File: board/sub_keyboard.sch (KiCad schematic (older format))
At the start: 30 parts, among them SW1001 SW_SPST, SW1002 SW_SPST, SW1003 SW_SPST, SW1004 SW_SPST, SW1005 SW_SPST, SW1006 SW_SPST, SW1007 SW_SPST, SW1008 SW_SPST, SW1009 SW_SPST, SW1010 SW_SPST, SW1011 SW_SPST, SW1012 SW_SPST, SW1013 SW_SPST, SW1014 SW_SPST, SW1015 SW_SPST, SW1016 SW_SPST, SW1017 SW_SPST, SW1018 SW_SPST, SW1019 SW_SPST, SW1020 SW_SPST, SW1021 SW_SPST, SW1022 SW_SPST, SW1023 SW_SPST, SW1024 SW_SPST, SW1025 SW_SPST, SW1026 SW_SPST, SW1027 SW_SPST, SW1028 SW_SPST, SW1029 SW_SPST, SW1030 SW_SPST

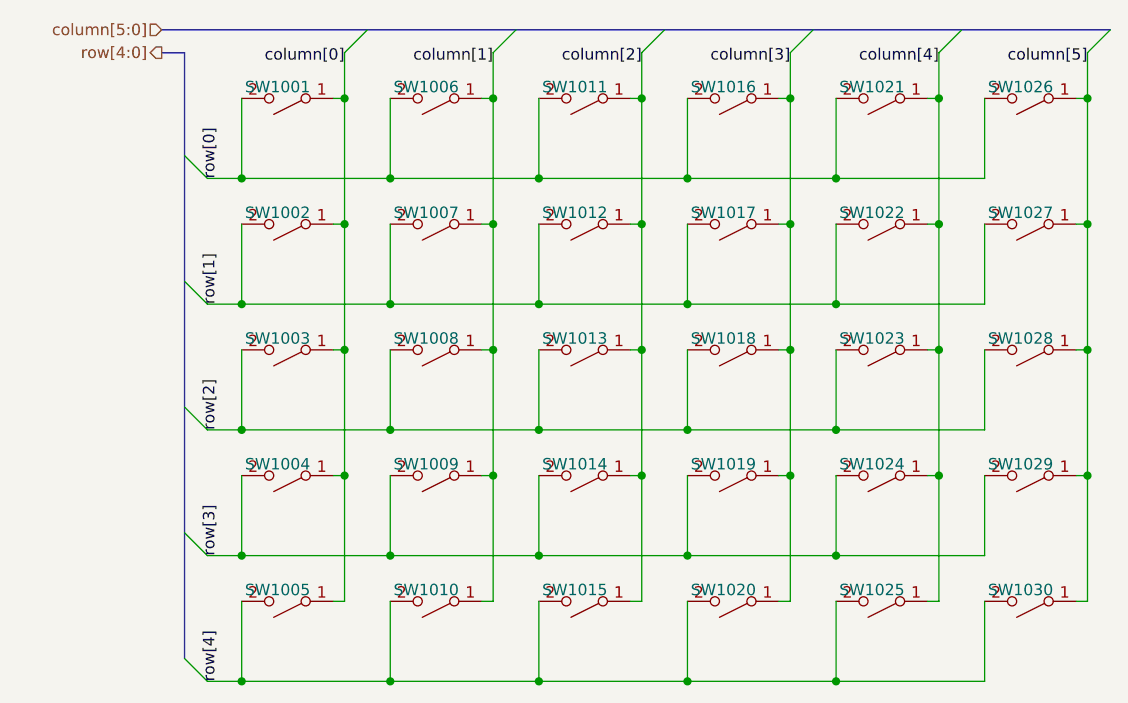
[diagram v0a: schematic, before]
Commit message: More Schematic progress
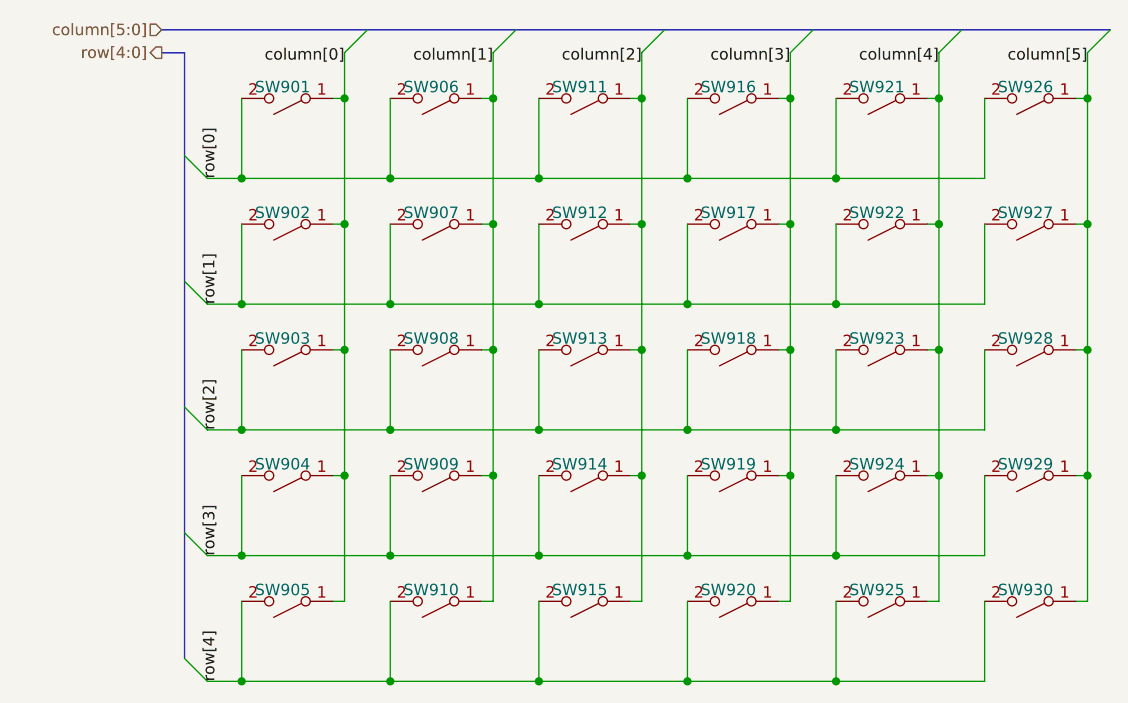
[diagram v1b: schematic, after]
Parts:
- renumbered SW1001 to SW901, SW1002 to SW902, SW1003 to SW903, SW1004 to SW904, SW1005 to SW905, SW1006 to SW906, SW1007 to SW907, SW1008 to SW908, SW1009 to SW909, SW1010 to SW910, SW1011 to SW911, SW1012 to SW912, SW1013 to SW913, SW1014 to SW914, SW1015 to SW915, SW1016 to SW916, SW1017 to SW917, SW1018 to SW918, SW1019 to SW919, SW1020 to SW920, SW1021 to SW921, SW1022 to SW922, SW1023 to SW923, SW1024 to SW924, SW1025 to SW925, SW1026 to SW926, SW1027 to SW927, SW1028 to SW928, SW1029 to SW929, SW1030 to SW930
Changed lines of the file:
@@
 $Descr A4 11693 8268
 encoding utf-8
-Sheet 10 15
+Sheet 9 14
 Title ""
 Date ""
@@
 row[4:0]
 $Comp
-L Switch:SW_SPST SW1001
+L Switch:SW_SPST SW901
 U 1 1 5A9DE7BF
 P 4600 2500
-F 0 "SW1001" H 4500 2450 50  0000 L CNN
+F 0 "SW901" H 4500 2450 50  0000 L CNN
 F 1 "SW_SPST" H 4450 2350 50  0001 L CNN
 F 2 "" H 4600 2500 50  0001 C CNN
@@
 $EndComp
 $Comp
-L Switch:SW_SPST SW1006
+L Switch:SW_SPST SW906
 U 1 1 5A9F6D51
 P 5250 2500
-F 0 "SW1006" H 5150 2450 50  0000 L CNN
+F 0 "SW906" H 5150 2450 50  0000 L CNN
 F 1 "SW_SPST" H 5100 2350 50  0001 L CNN
 F 2 "" H 5250 2500 50  0001 C CNN
@@
 $EndComp
 $Comp
-L Switch:SW_SPST SW1011
+L Switch:SW_SPST SW911
 U 1 1 5A9F724F
 P 5900 2500
-F 0 "SW1011" H 5800 2450 50  0000 L CNN
+F 0 "SW911" H 5800 2450 50  0000 L CNN
 F 1 "SW_SPST" H 5750 2350 50  0001 L CNN
 F 2 "" H 5900 2500 50  0001 C CNN
@@
 $EndComp
 $Comp
-L Switch:SW_SPST SW1016
+L Switch:SW_SPST SW916
 U 1 1 5A9F725B
 P 6550 2500
-F 0 "SW1016" H 6450 2450 50  0000 L CNN
+F 0 "SW916" H 6450 2450 50  0000 L CNN
 F 1 "SW_SPST" H 6400 2350 50  0001 L CNN
 F 2 "" H 6550 2500 50  0001 C CNN
@@
 $EndComp
 $Comp
-L Switch:SW_SPST SW1021
+L Switch:SW_SPST SW921
 U 1 1 5A9F738F
 P 7200 2500
-F 0 "SW1021" H 7100 2450 50  0000 L CNN
+F 0 "SW921" H 7100 2450 50  0000 L CNN
 F 1 "SW_SPST" H 7050 2350 50  0001 L CNN
 F 2 "" H 7200 2500 50  0001 C CNN
@@
 $EndComp
 $Comp
-L Switch:SW_SPST SW1026
+L Switch:SW_SPST SW926
 U 1 1 5A9F739B
 P 7850 2500
-F 0 "SW1026" H 7750 2450 50  0000 L CNN
+F 0 "SW926" H 7750 2450 50  0000 L CNN
 F 1 "SW_SPST" H 7700 2350 50  0001 L CNN
 F 2 "" H 7850 2500 50  0001 C CNN
@@
 $EndComp
 $Comp
-L Switch:SW_SPST SW1002
+L Switch:SW_SPST SW902
 U 1 1 5A9F7527
 P 4600 3050
-F 0 "SW1002" H 4500 3000 50  0000 L CNN
+F 0 "SW902" H 4500 3000 50  0000 L CNN
 F 1 "SW_SPST" H 4450 2900 50  0001 L CNN
 F 2 "" H 4600 3050 50  0001 C CNN
@@
 $EndComp
 $Comp
-L Switch:SW_SPST SW1007
+L Switch:SW_SPST SW907
 U 1 1 5A9F7533
 P 5250 3050
-F 0 "SW1007" H 5150 3000 50  0000 L CNN
+F 0 "SW907" H 5150 3000 50  0000 L CNN
 F 1 "SW_SPST" H 5100 2900 50  0001 L CNN
 F 2 "" H 5250 3050 50  0001 C CNN
@@
 $EndComp
 $Comp
-L Switch:SW_SPST SW1012
+L Switch:SW_SPST SW912
 U 1 1 5A9F753F
 P 5900 3050
-F 0 "SW1012" H 5800 3000 50  0000 L CNN
+F 0 "SW912" H 5800 3000 50  0000 L CNN
 F 1 "SW_SPST" H 5750 2900 50  0001 L CNN
 F 2 "" H 5900 3050 50  0001 C CNN
@@
 $EndComp
 $Comp
-L Switch:SW_SPST SW1017
+L Switch:SW_SPST SW917
 U 1 1 5A9F754B
 P 6550 3050
-F 0 "SW1017" H 6450 3000 50  0000 L CNN
+F 0 "SW917" H 6450 3000 50  0000 L CNN
 F 1 "SW_SPST" H 6400 2900 50  0001 L CNN
 F 2 "" H 6550 3050 50  0001 C CNN
@@
 $EndComp
 $Comp
-L Switch:SW_SPST SW1022
+L Switch:SW_SPST SW922
 U 1 1 5A9F7557
 P 7200 3050
-F 0 "SW1022" H 7100 3000 50  0000 L CNN
+F 0 "SW922" H 7100 3000 50  0000 L CNN
 F 1 "SW_SPST" H 7050 2900 50  0001 L CNN
 F 2 "" H 7200 3050 50  0001 C CNN
@@
 $EndComp
 $Comp
-L Switch:SW_SPST SW1027
+L Switch:SW_SPST SW927
 U 1 1 5A9F7563
 P 7850 3050
-F 0 "SW1027" H 7750 3000 50  0000 L CNN
+F 0 "SW927" H 7750 3000 50  0000 L CNN
 F 1 "SW_SPST" H 7700 2900 50  0001 L CNN
 F 2 "" H 7850 3050 50  0001 C CNN
@@
 $EndComp
 $Comp
-L Switch:SW_SPST SW1003
+L Switch:SW_SPST SW903
 U 1 1 5A9F8C97
 P 4600 3600
-F 0 "SW1003" H 4500 3550 50  0000 L CNN
+F 0 "SW903" H 4500 3550 50  0000 L CNN
 F 1 "SW_SPST" H 4450 3450 50  0001 L CNN
 F 2 "" H 4600 3600 50  0001 C CNN
@@
 $EndComp
 $Comp
-L Switch:SW_SPST SW1008
+L Switch:SW_SPST SW908
 U 1 1 5A9F8CA3
 P 5250 3600
-F 0 "SW1008" H 5150 3550 50  0000 L CNN
+F 0 "SW908" H 5150 3550 50  0000 L CNN
 F 1 "SW_SPST" H 5100 3450 50  0001 L CNN
 F 2 "" H 5250 3600 50  0001 C CNN
@@
 $EndComp
 $Comp
-L Switch:SW_SPST SW1013
+L Switch:SW_SPST SW913
 U 1 1 5A9F8CAF
 P 5900 3600
-F 0 "SW1013" H 5800 3550 50  0000 L CNN
+F 0 "SW913" H 5800 3550 50  0000 L CNN
 F 1 "SW_SPST" H 5750 3450 50  0001 L CNN
 F 2 "" H 5900 3600 50  0001 C CNN
@@
 $EndComp
 $Comp
-L Switch:SW_SPST SW1018
+L Switch:SW_SPST SW918
 U 1 1 5A9F8CBB
 P 6550 3600
-F 0 "SW1018" H 6450 3550 50  0000 L CNN
+F 0 "SW918" H 6450 3550 50  0000 L CNN
 F 1 "SW_SPST" H 6400 3450 50  0001 L CNN
 F 2 "" H 6550 3600 50  0001 C CNN
@@
 $EndComp
 $Comp
-L Switch:SW_SPST SW1023
+L Switch:SW_SPST SW923
 U 1 1 5A9F8CC7
 P 7200 3600
-F 0 "SW1023" H 7100 3550 50  0000 L CNN
+F 0 "SW923" H 7100 3550 50  0000 L CNN
 F 1 "SW_SPST" H 7050 3450 50  0001 L CNN
 F 2 "" H 7200 3600 50  0001 C CNN
@@
 $EndComp
 $Comp
-L Switch:SW_SPST SW1028
+L Switch:SW_SPST SW928
 U 1 1 5A9F8CD3
 P 7850 3600
-F 0 "SW1028" H 7750 3550 50  0000 L CNN
+F 0 "SW928" H 7750 3550 50  0000 L CNN
 F 1 "SW_SPST" H 7700 3450 50  0001 L CNN
 F 2 "" H 7850 3600 50  0001 C CNN
@@
 $EndComp
 $Comp
-L Switch:SW_SPST SW1004
+L Switch:SW_SPST SW904
 U 1 1 5A9F94D7
 P 4600 4150
-F 0 "SW1004" H 4500 4100 50  0000 L CNN
+F 0 "SW904" H 4500 4100 50  0000 L CNN
 F 1 "SW_SPST" H 4450 4000 50  0001 L CNN
 F 2 "" H 4600 4150 50  0001 C CNN
@@
 $EndComp
 $Comp
-L Switch:SW_SPST SW1009
+L Switch:SW_SPST SW909
 U 1 1 5A9F94E3
 P 5250 4150
-F 0 "SW1009" H 5150 4100 50  0000 L CNN
+F 0 "SW909" H 5150 4100 50  0000 L CNN
 F 1 "SW_SPST" H 5100 4000 50  0001 L CNN
 F 2 "" H 5250 4150 50  0001 C CNN
@@
 $EndComp
 $Comp
-L Switch:SW_SPST SW1014
+L Switch:SW_SPST SW914
 U 1 1 5A9F94EF
 P 5900 4150
-F 0 "SW1014" H 5800 4100 50  0000 L CNN
+F 0 "SW914" H 5800 4100 50  0000 L CNN
 F 1 "SW_SPST" H 5750 4000 50  0001 L CNN
 F 2 "" H 5900 4150 50  0001 C CNN
@@
 $EndComp
 $Comp
-L Switch:SW_SPST SW1019
+L Switch:SW_SPST SW919
 U 1 1 5A9F94FB
 P 6550 4150
-F 0 "SW1019" H 6450 4100 50  0000 L CNN
+F 0 "SW919" H 6450 4100 50  0000 L CNN
 F 1 "SW_SPST" H 6400 4000 50  0001 L CNN
 F 2 "" H 6550 4150 50  0001 C CNN
@@
 $EndComp
 $Comp
-L Switch:SW_SPST SW1024
+L Switch:SW_SPST SW924
 U 1 1 5A9F9507
 P 7200 4150
-F 0 "SW1024" H 7100 4100 50  0000 L CNN
+F 0 "SW924" H 7100 4100 50  0000 L CNN
 F 1 "SW_SPST" H 7050 4000 50  0001 L CNN
 F 2 "" H 7200 4150 50  0001 C CNN
@@
 $EndComp
 $Comp
-L Switch:SW_SPST SW1029
+L Switch:SW_SPST SW929
 U 1 1 5A9F9513
 P 7850 4150
-F 0 "SW1029" H 7750 4100 50  0000 L CNN
+F 0 "SW929" H 7750 4100 50  0000 L CNN
 F 1 "SW_SPST" H 7700 4000 50  0001 L CNN
 F 2 "" H 7850 4150 50  0001 C CNN
@@
 $EndComp
 $Comp
-L Switch:SW_SPST SW1005
+L Switch:SW_SPST SW905
 U 1 1 5A9F951F
 P 4600 4700
-F 0 "SW1005" H 4500 4650 50  0000 L CNN
+F 0 "SW905" H 4500 4650 50  0000 L CNN
 F 1 "SW_SPST" H 4450 4550 50  0001 L CNN
 F 2 "" H 4600 4700 50  0001 C CNN
@@
 $EndComp
 $Comp
-L Switch:SW_SPST SW1010
+L Switch:SW_SPST SW910
 U 1 1 5A9F952B
 P 5250 4700
-F 0 "SW1010" H 5150 4650 50  0000 L CNN
+F 0 "SW910" H 5150 4650 50  0000 L CNN
 F 1 "SW_SPST" H 5100 4550 50  0001 L CNN
 F 2 "" H 5250 4700 50  0001 C CNN
@@
 $EndComp
 $Comp
-L Switch:SW_SPST SW1015
+L Switch:SW_SPST SW915
 U 1 1 5A9F9537
 P 5900 4700
-F 0 "SW1015" H 5800 4650 50  0000 L CNN
+F 0 "SW915" H 5800 4650 50  0000 L CNN
 F 1 "SW_SPST" H 5750 4550 50  0001 L CNN
 F 2 "" H 5900 4700 50  0001 C CNN
@@
 $EndComp
 $Comp
-L Switch:SW_SPST SW1020
+L Switch:SW_SPST SW920
 U 1 1 5A9F9543
 P 6550 4700
-F 0 "SW1020" H 6450 4650 50  0000 L CNN
+F 0 "SW920" H 6450 4650 50  0000 L CNN
 F 1 "SW_SPST" H 6400 4550 50  0001 L CNN
 F 2 "" H 6550 4700 50  0001 C CNN
@@
 $EndComp
 $Comp
-L Switch:SW_SPST SW1025
+L Switch:SW_SPST SW925
 U 1 1 5A9F954F
 P 7200 4700
-F 0 "SW1025" H 7100 4650 50  0000 L CNN
+F 0 "SW925" H 7100 4650 50  0000 L CNN
 F 1 "SW_SPST" H 7050 4550 50  0001 L CNN
 F 2 "" H 7200 4700 50  0001 C CNN
@@
 $EndComp
 $Comp
-L Switch:SW_SPST SW1030
+L Switch:SW_SPST SW930
 U 1 1 5A9F955B
 P 7850 4700
-F 0 "SW1030" H 7750 4650 50  0000 L CNN
+F 0 "SW930" H 7750 4650 50  0000 L CNN
 F 1 "SW_SPST" H 7700 4550 50  0001 L CNN
 F 2 "" H 7850 4700 50  0001 C CNN
